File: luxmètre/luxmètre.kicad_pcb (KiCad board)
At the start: 4 copper layers, 108.9 x 64.9 mm, 110 parts, among them J1 Conn_01x01, J10 Conn_01x01, J11 Conn_01x01, J12 Conn_01x01, J13 Conn_01x01, J14 Conn_01x01, J15 Conn_01x03, J16 Conn_01x03, J2 Conn_01x01, J3 USB_A, J4 Conn_01x01, J5 Conn_01x04, J6 Conn_01x08, J7 Conn_01x08, J8 Conn_01x10, J9 Conn_01x03, SW1 B3S-1000P, SW2 SW_DIP_x01, U1 ILB1206ER260V, U10 RF-LORA-868-SO, U11 AD8418, U12 MCP73831-2-MC, U13 ADC-10-4+, U2 ILB1206ER260V, U3 ILB1206ER260V, U4 ESP32-WROOM-32, U5 FT232HL, U7 PCA9537DP, U8 MAX1674EUA+T, U9 LM1117MP-3.3, Y1 12MHz

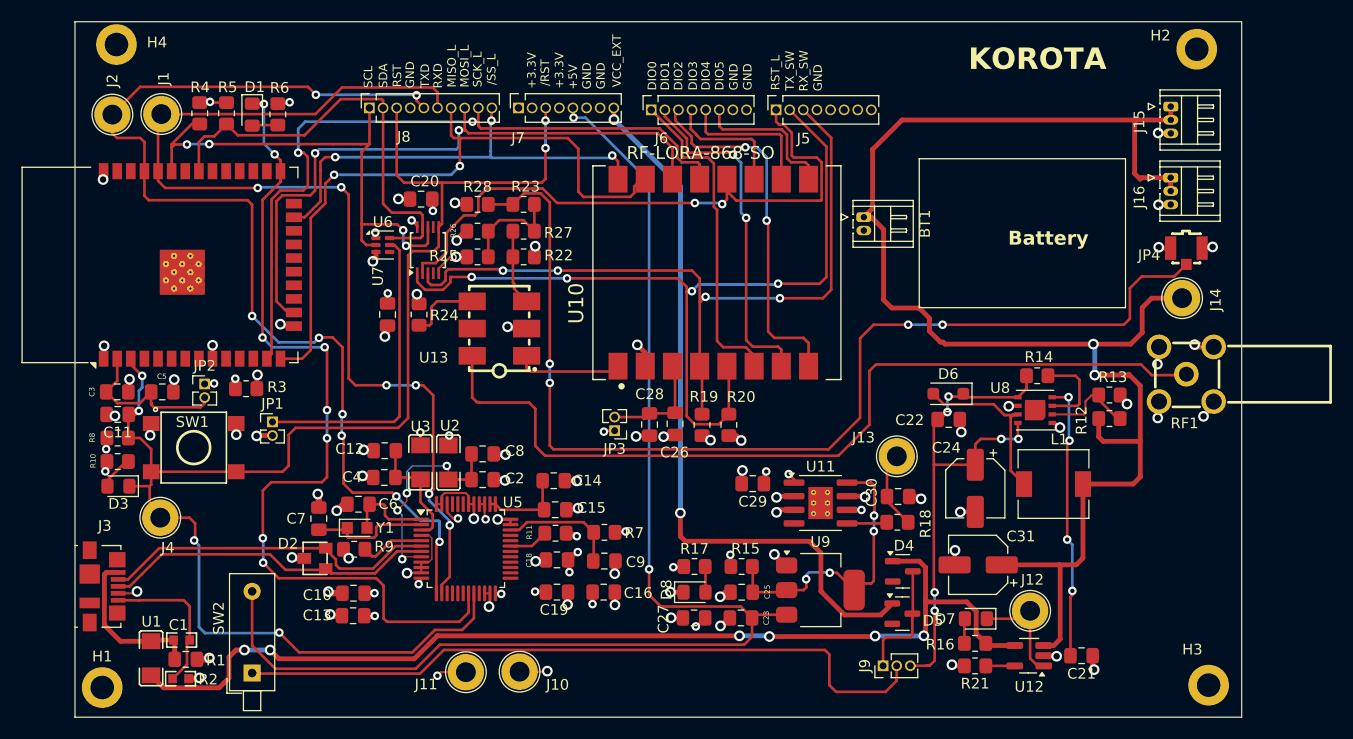
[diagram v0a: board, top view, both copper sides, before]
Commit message: pcb
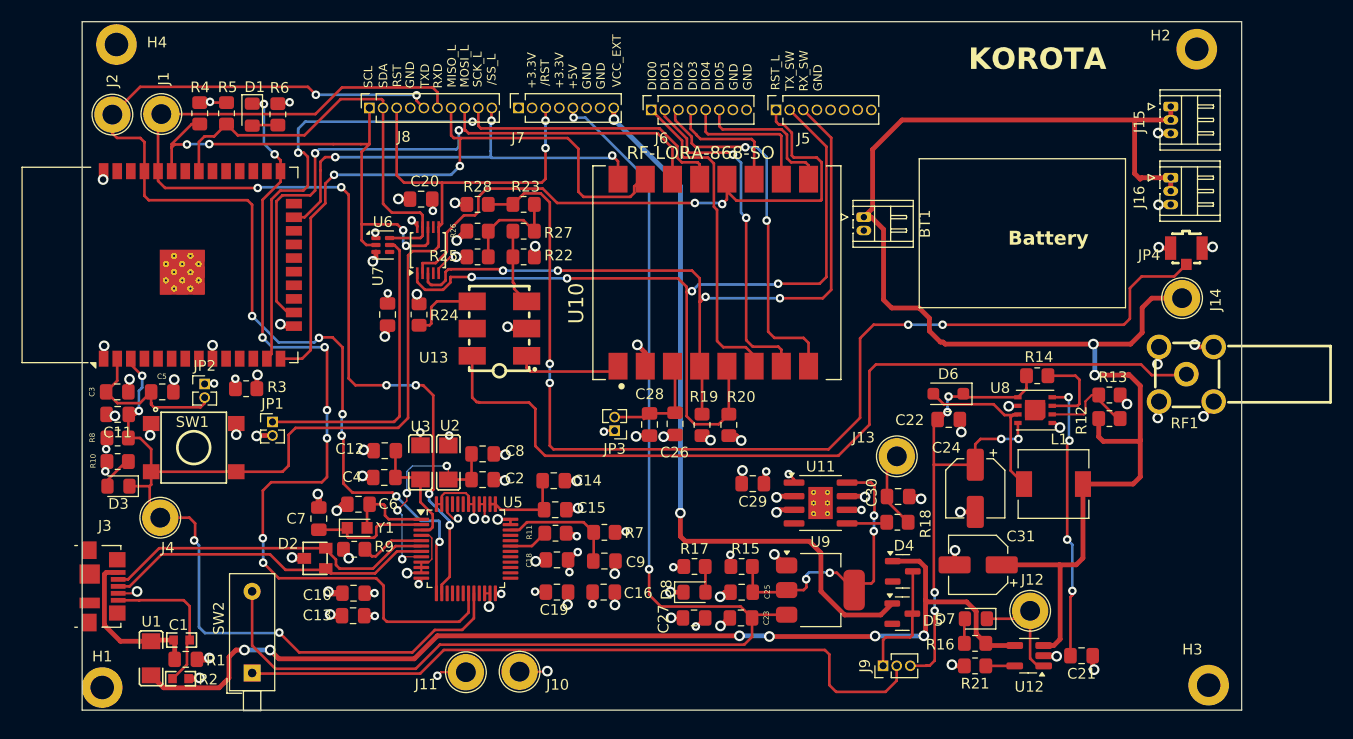
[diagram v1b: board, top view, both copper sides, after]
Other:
- board size 108.9 x 64.9 mm -> 108.2 x 64.2 mm
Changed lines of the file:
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@@
 			(outputformat 1)
 			(mirror no)
-			(drillshape 1)
+			(drillshape 0)
 			(scaleselection 1)
 			(outputdirectory "")
@@
 	)
 	(gr_rect
-		(start 48.63 41.75)
-		(end 157.51 106.66)
+		(start 49.3 41.75)
+		(end 157.51 106)
 		(stroke
 			(width 0.05)
@@
 		(polygon
 			(pts
-				(xy 49.82 45.69) (xy 158.42 45.5) (xy 158.21 104.88) (xy 49.58 105.29)
+				(xy 48.42 41.69) (xy 157.02 41.5) (xy 158.51 105.98) (xy 49.88 106.39)
 			)
 		)
@@
 		(polygon
 			(pts
-				(xy 49.6 46.42) (xy 158.63 45.55) (xy 157.98 104.37) (xy 49.57 105.25)
+				(xy 49 42.12) (xy 158.03 41.25) (xy 157.78 105.67) (xy 49.37 106.55)
 			)
 		)
